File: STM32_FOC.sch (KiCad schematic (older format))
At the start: 46 parts, among them J1 Conn_01x07, J2 Conn_01x02, J3 Conn_01x03, J4 Conn_01x04, U1 STM32F103C8T6, U2 MP2359, U3 AS5600, U4 DRV8313, Y1 Crystal_GND3_Small

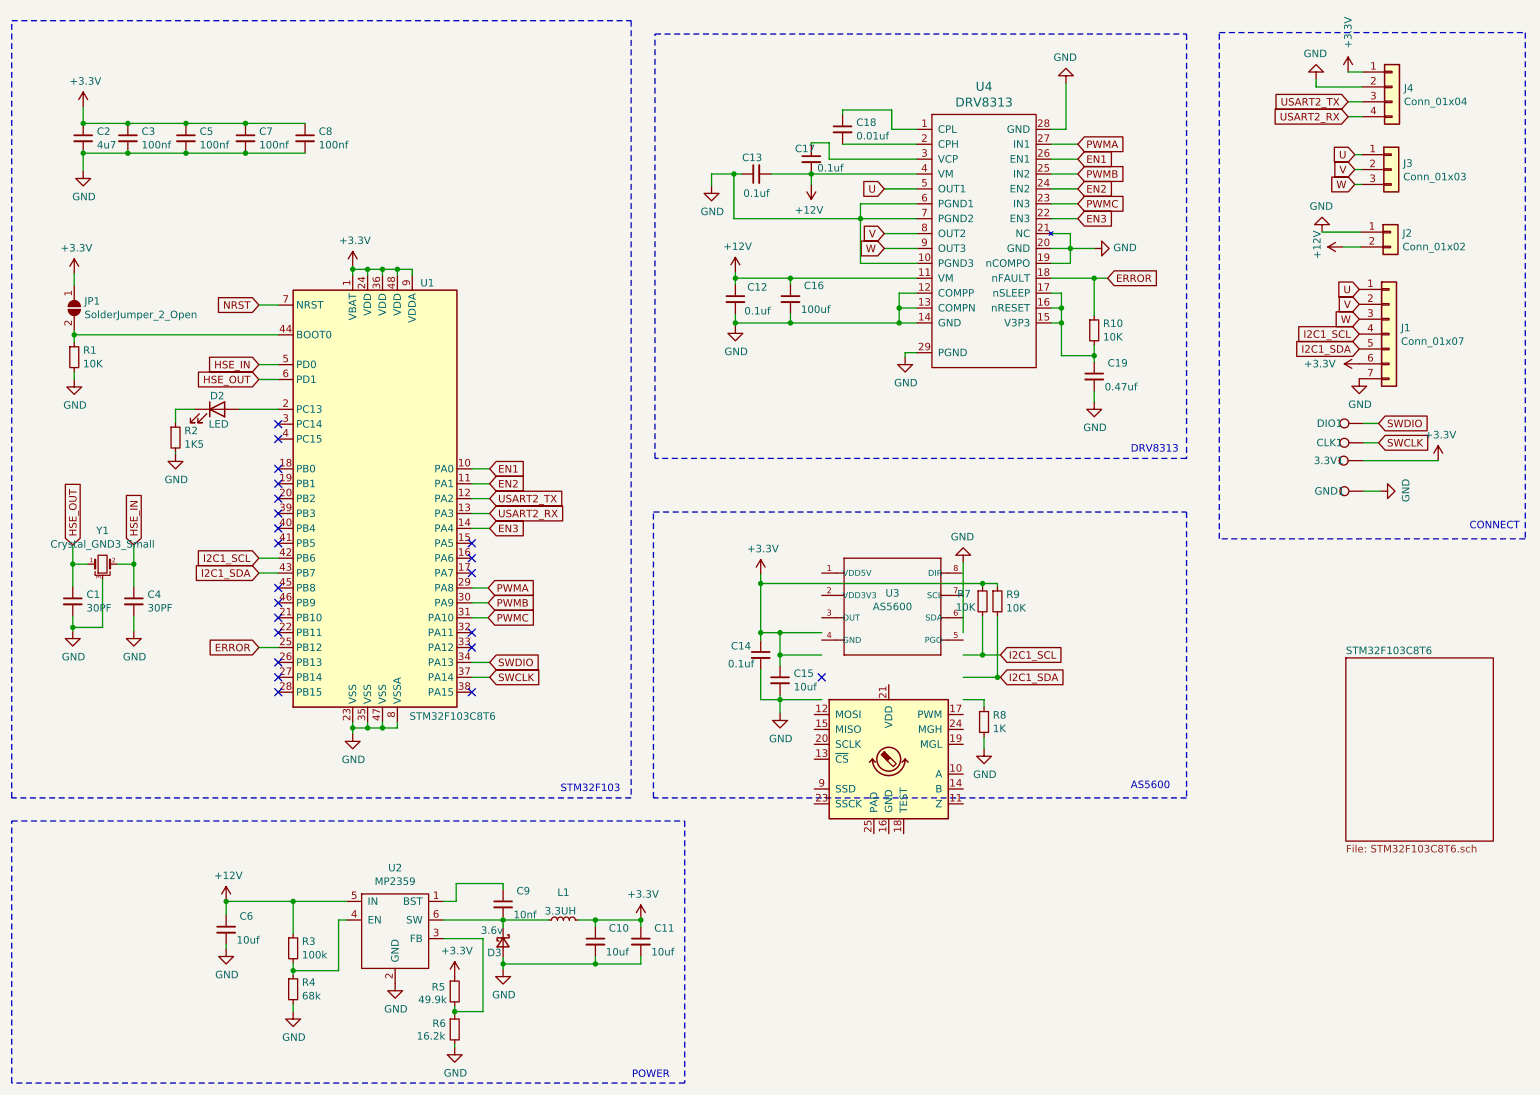
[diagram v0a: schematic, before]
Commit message: first commit
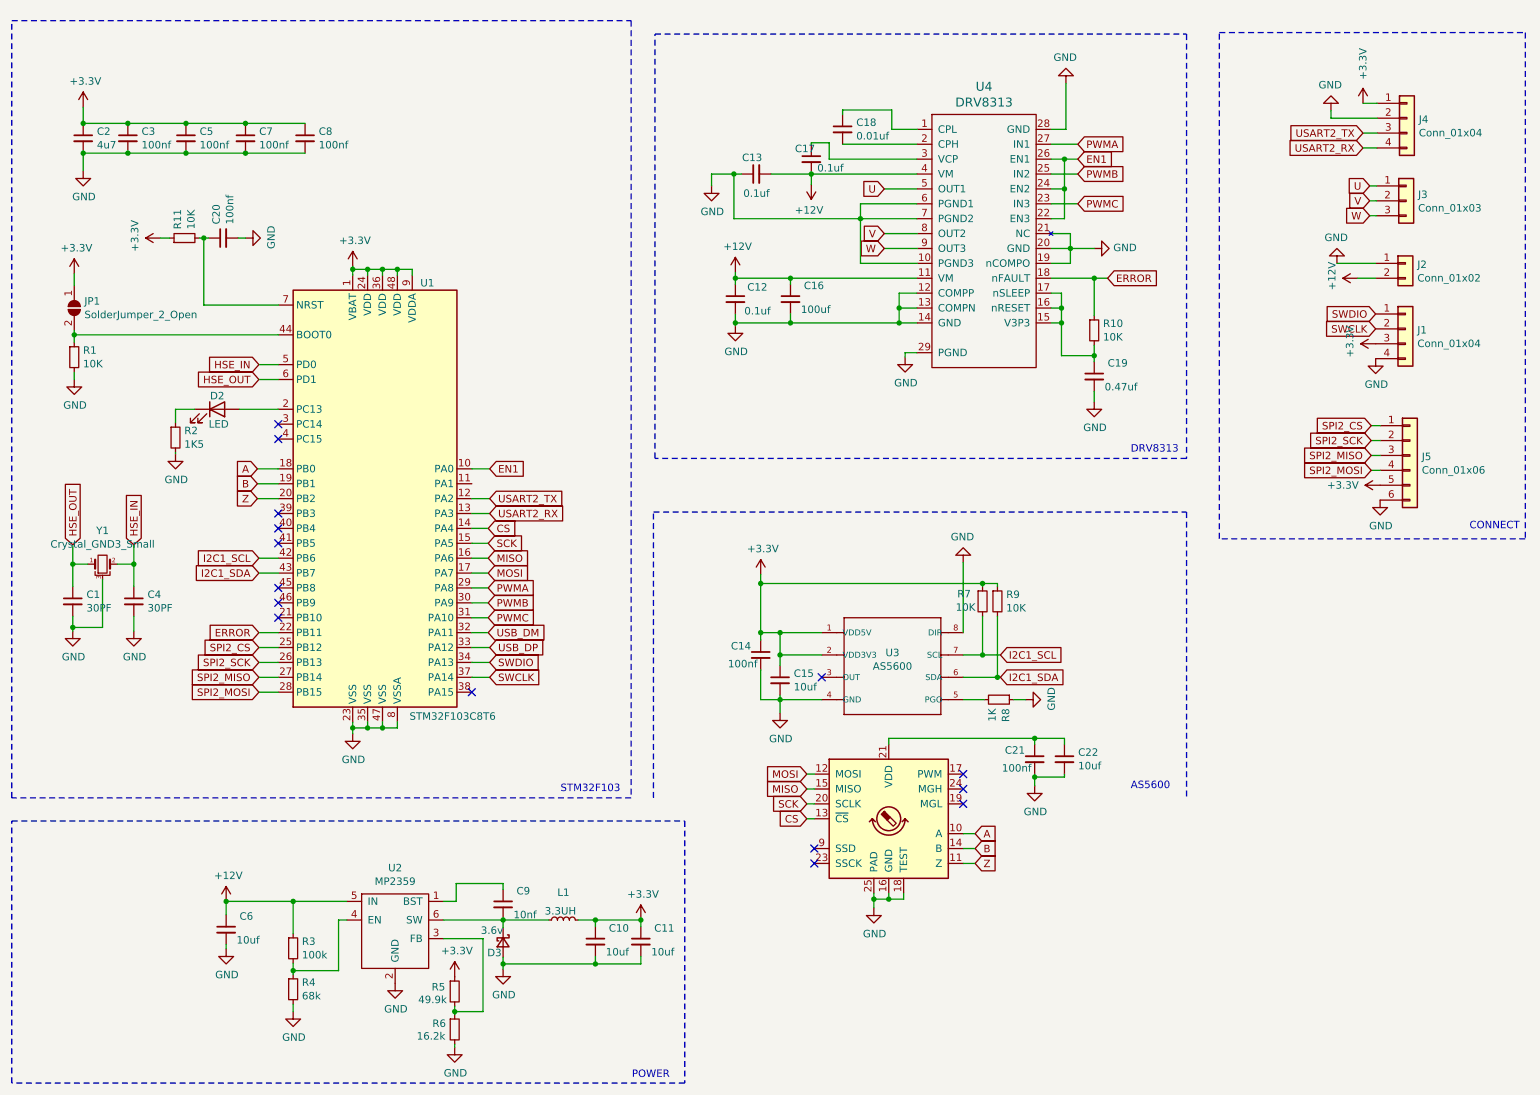
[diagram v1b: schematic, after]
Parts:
- removed 3.3V1, CLK1, DIO1, GND1: TestPoint, TestPoint:TestPoint_Pad_D1.0mm, symbol Connector:TestPoint
- removed J1: Conn_01x07, Connector_JST:JST_SH_SM07B-SRSS-TB_1x07-1MP_P1.00mm_Horizontal, symbol Connector_Generic:Conn_01x07
- added C20, C21: 100nf, Capacitor_SMD:C_0402_1005Metric, symbol Device:C_Small
- added C22: 10uf, Capacitor_SMD:C_0603_1608Metric, symbol Device:C_Small
- added J1: Conn_01x04, Connector_JST:JST_SH_SM04B-SRSS-TB_1x04-1MP_P1.00mm_Horizontal, symbol Connector_Generic:Conn_01x04
- added J5: Conn_01x06, Connector_JST:JST_SH_SM06B-SRSS-TB_1x06-1MP_P1.00mm_Horizontal, symbol Connector_Generic:Conn_01x06
- added R11: 10K, Resistor_SMD:R_0402_1005Metric, symbol Device:R_Small
- C1, C10, C11, C12, C13, C16, C17, C18, C19, C2, C3, C4, C5, C7, C8, C9: footprint Capacitor_SMD:C_0603_1608Metric -> Capacitor_SMD:C_0402_1005Metric
- C14: value 0.1uf -> 100nf; footprint Capacitor_SMD:C_0603_1608Metric -> Capacitor_SMD:C_0402_1005Metric
- D2: footprint LED_SMD:LED_0603_1608Metric -> LED_SMD:LED_0402_1005Metric
- JP1: footprint Jumper:SolderJumper-2_P1.3mm_Open_RoundedPad1.0x1.5mm -> Jumper:SoldJumper-2-P0.5mm_Open_RoundedPad
- R1, R10, R2, R3, R4, R5, R6, R7, R8, R9: footprint Resistor_SMD:R_0603_1608Metric -> Resistor_SMD:R_0402_1005Metric
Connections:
- net labels added: A, B, CS, MISO, MOSI, SCK, SPI2_CS, SPI2_MISO, SPI2_MOSI, SPI2_SCK, USB_DM, USB_DP, Z
- net labels removed: EN2, EN3, NRST
- wire segments 209 -> 249
- no-connect marks 22 -> 15
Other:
- moved on the sheet: J2, J3, J4, R8, U3

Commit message: updata
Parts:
- C12: footprint Capacitor_SMD:C_0402_1005Metric -> Capacitor_SMD:C_0603_1608Metric
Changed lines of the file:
@@
 F 0 "C12" H 5580 2530 50  0000 L CNN
 F 1 "0.1uf" H 5560 2370 50  0000 L CNN
-F 2 "Capacitor_SMD:C_0402_1005Metric" H 5500 2450 50  0001 C CNN
+F 2 "Capacitor_SMD:C_0603_1608Metric" H 5500 2450 50  0001 C CNN
 F 3 "~" H 5500 2450 50  0001 C CNN
 	1    5500 2450
